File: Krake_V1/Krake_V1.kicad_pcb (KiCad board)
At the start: 4 copper layers, 107.5 x 102 mm, 60 parts, among them J1 Barrel_Jack_Switch_SMT, Q1 BSS138, U1 LM7805_TO220, U2 PCF8574AT_3_518, U3 LCD_20x4_Character-GPAD_SCH_L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

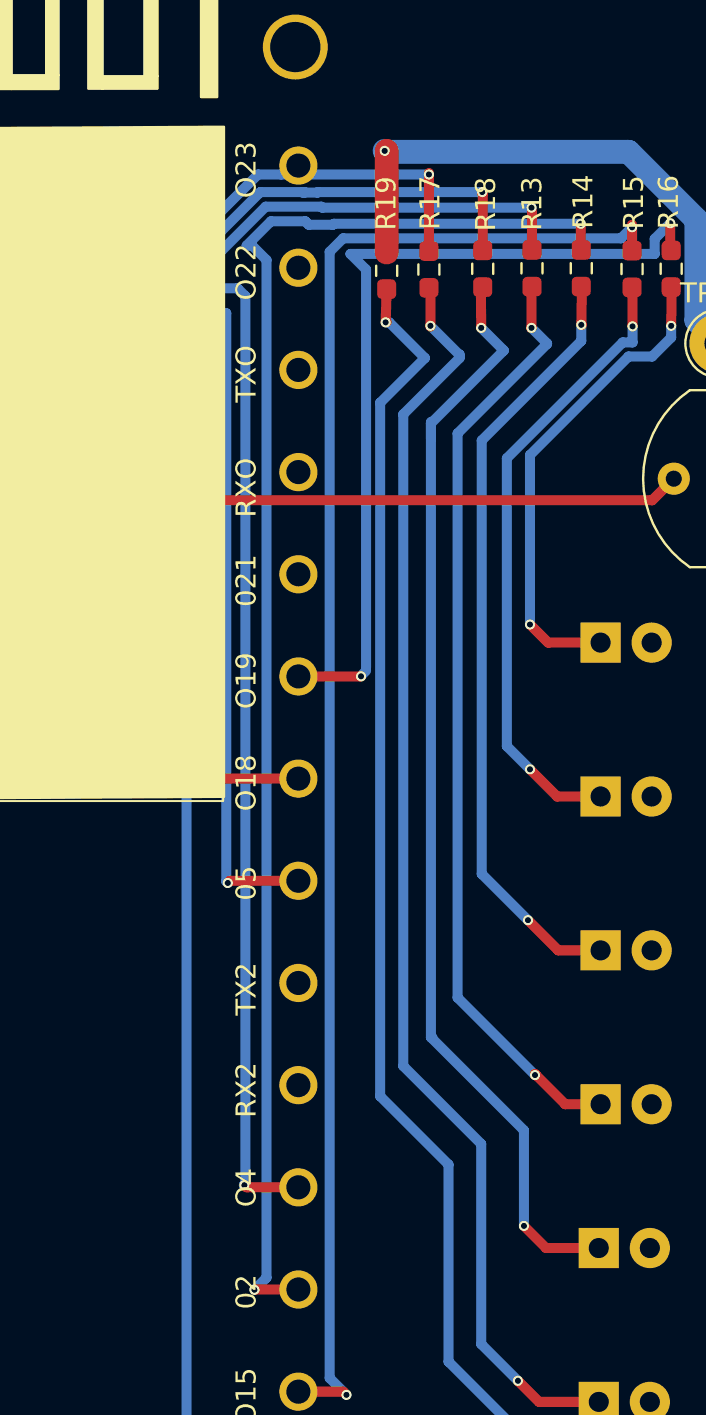
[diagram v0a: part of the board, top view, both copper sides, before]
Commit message: Placed the files for LCD debugging in a factory test file.
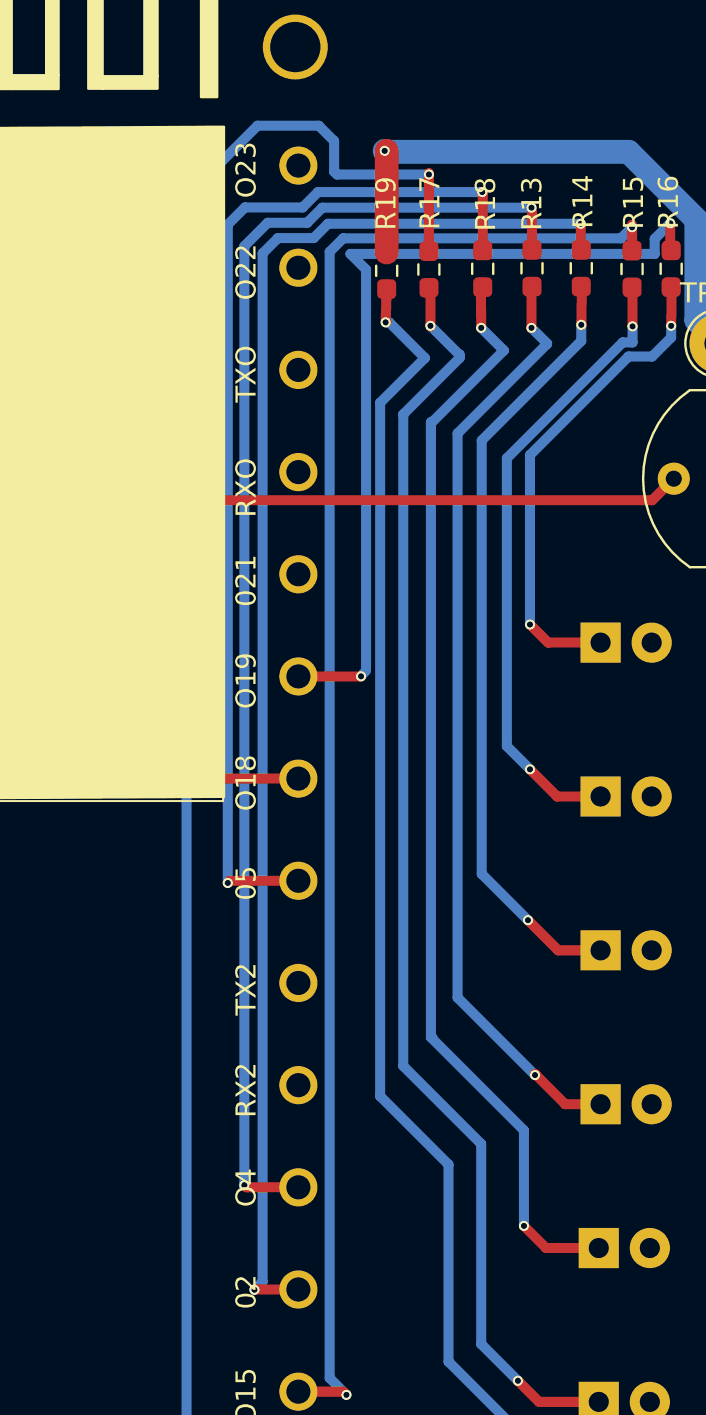
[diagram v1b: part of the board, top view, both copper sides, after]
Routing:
- net Net-(ESP1-O4): track 71.1 -> 66.5 mm
- net Net-(ESP1-O5): track 57.1 -> 52.5 mm
- net Net-(ESP1-O2): track 73.4 -> 71.6 mm
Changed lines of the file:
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@@
   (via (at 202.325 34.175) (size 0.5) (drill 0.3) (layers "F.Cu" "B.Cu") (net 31))
   (via (at 191 63.9) (size 0.5) (drill 0.3) (layers "F.Cu" "B.Cu") (net 31))
-  (segment (start 202.325 34.175) (end 194.975 34.175) (width 0.5) (layer "B.Cu") (net 31))
-  (segment (start 190.975 63.875) (end 191 63.9) (width 0.5) (layer "B.Cu") (net 31))
-  (segment (start 187.25 40.875) (end 188.55 42.175) (width 0.5) (layer "B.Cu") (net 31))
-  (segment (start 194.975 34.175) (end 193.828079 34.175) (width 0.5) (layer "B.Cu") (net 31))
-  (segment (start 190.975 42.5) (end 190.975 63.875) (width 0.5) (layer "B.Cu") (net 31))
-  (segment (start 188.875 42.5) (end 190.975 42.5) (width 0.5) (layer "B.Cu") (net 31))
-  (segment (start 188.55 42.175) (end 188.875 42.5) (width 0.5) (layer "B.Cu") (net 31))
-  (segment (start 193.828079 34.175) (end 187.25 40.753079) (width 0.5) (layer "B.Cu") (net 31))
-  (segment (start 187.25 40.753079) (end 187.25 40.875) (width 0.5) (layer "B.Cu") (net 31))
+  (segment (start 197.612 32.512) (end 196.85 31.75) (width 0.5) (layer "B.Cu") (net 31))
+  (segment (start 193.802 31.75) (end 191.625 33.927) (width 0.5) (layer "B.Cu") (net 31))
+  (segment (start 197.612 34.036) (end 197.612 32.512) (width 0.5) (layer "B.Cu") (net 31))
+  (segment (start 196.85 31.75) (end 193.802 31.75) (width 0.5) (layer "B.Cu") (net 31))
+  (segment (start 197.751 34.175) (end 197.612 34.036) (width 0.5) (layer "B.Cu") (net 31))
+  (segment (start 191.625 63.275) (end 191 63.9) (width 0.5) (layer "B.Cu") (net 31))
+  (segment (start 202.325 34.175) (end 197.751 34.175) (width 0.5) (layer "B.Cu") (net 31))
+  (segment (start 191.625 33.927) (end 191.625 63.275) (width 0.5) (layer "B.Cu") (net 31))
   (segment (start 195.835 69.2916) (end 192.4334 69.2916) (width 0.5) (layer "F.Cu") (net 32))
   (segment (start 192.4334 69.2916) (end 192.325 69.4) (width 0.5) (layer "F.Cu") (net 32))
@@
   (via (at 192.325 69.4) (size 0.5) (drill 0.3) (layers "F.Cu" "B.Cu") (net 32))
   (via (at 204.975 35.05) (size 0.5) (drill 0.3) (layers "F.Cu" "B.Cu") (net 32))
-  (segment (start 189.731971 41.075) (end 192.25 41.075) (width 0.5) (layer "B.Cu") (net 32))
-  (segment (start 192.25 69.325) (end 192.325 69.4) (width 0.5) (layer "B.Cu") (net 32))
-  (segment (start 196.125 35.075) (end 196.15 35.05) (width 0.5) (layer "B.Cu") (net 32))
-  (segment (start 196.810051 35.05) (end 196.785051 35.075) (width 0.5) (layer "B.Cu") (net 32))
-  (segment (start 193.943029 35.05) (end 188.825 40.168029) (width 0.5) (layer "B.Cu") (net 32))
-  (segment (start 196.785051 35.075) (end 196.05 35.075) (width 0.5) (layer "B.Cu") (net 32))
-  (segment (start 188.825 40.168029) (end 189.731971 41.075) (width 0.5) (layer "B.Cu") (net 32))
-  (segment (start 196.15 35.05) (end 193.943029 35.05) (width 0.5) (layer "B.Cu") (net 32))
+  (segment (start 196.810051 35.05) (end 196.046051 35.814) (width 0.5) (layer "B.Cu") (net 32))
+  (segment (start 196.046051 35.814) (end 193.179029 35.814) (width 0.5) (layer "B.Cu") (net 32))
+  (segment (start 192.325 36.668029) (end 192.325 69.4) (width 0.5) (layer "B.Cu") (net 32))
   (segment (start 204.975 35.05) (end 196.810051 35.05) (width 0.5) (layer "B.Cu") (net 32))
-  (segment (start 196.05 35.075) (end 196.125 35.075) (width 0.5) (layer "B.Cu") (net 32))
-  (segment (start 192.25 41.075) (end 192.25 69.325) (width 0.5) (layer "B.Cu") (net 32))
+  (segment (start 193.179029 35.814) (end 192.325 36.668029) (width 0.5) (layer "B.Cu") (net 32))
   (segment (start 150.8 62.225) (end 148.45 62.225) (width 0.5) (layer "F.Cu") (net 34))
   (via (at 148.45 62.225) (size 0.5) (drill 0.3) (layers "F.Cu" "B.Cu") (net 34))
@@
   (via (at 207.425 35.825) (size 0.5) (drill 0.3) (layers "F.Cu" "B.Cu") (net 35))
   (via (at 193.15 84.425) (size 0.5) (drill 0.3) (layers "F.Cu" "B.Cu") (net 35))
-  (segment (start 190.15 39.832979) (end 192.807979 39.832979) (width 0.5) (layer "B.Cu") (net 35))
-  (segment (start 194.207979 35.775) (end 190.15 39.832979) (width 0.5) (layer "B.Cu") (net 35))
-  (segment (start 196.975 35.775) (end 194.207979 35.775) (width 0.5) (layer "B.Cu") (net 35))
+  (segment (start 193.15 37.736) (end 193.15 84.4) (width 0.5) (layer "B.Cu") (net 35))
+  (segment (start 194.31 36.576) (end 193.15 37.736) (width 0.5) (layer "B.Cu") (net 35))
+  (segment (start 207.425 35.825) (end 197.025 35.825) (width 0.5) (layer "B.Cu") (net 35))
   (segment (start 193.15 84.4) (end 193.15 84.425) (width 0.5) (layer "B.Cu") (net 35))
+  (segment (start 196.274 36.576) (end 194.31 36.576) (width 0.5) (layer "B.Cu") (net 35))
   (segment (start 193.15 84.425) (end 193.125 84.425) (width 0.5) (layer "B.Cu") (net 35))
-  (segment (start 193.2 40.225) (end 193.2 84.35) (width 0.5) (layer "B.Cu") (net 35))
-  (segment (start 193.2 84.35) (end 193.15 84.4) (width 0.5) (layer "B.Cu") (net 35))
-  (segment (start 207.425 35.825) (end 197.025 35.825) (width 0.5) (layer "B.Cu") (net 35))
-  (segment (start 192.807979 39.832979) (end 193.2 40.225) (width 0.5) (layer "B.Cu") (net 35))
+  (segment (start 197.025 35.825) (end 196.274 36.576) (width 0.5) (layer "B.Cu") (net 35))
   (segment (start 193.125 84.425) (end 193.15 84.4) (width 0.5) (layer "B.Cu") (net 35))
-  (segment (start 197.025 35.825) (end 196.975 35.775) (width 0.5) (layer "B.Cu") (net 35))
   (segment (start 209.9 37.925) (end 209.875 37.9) (width 0.5) (layer "F.Cu") (net 36))
   (segment (start 193.6634 89.6116) (end 193.65 89.625) (width 0.5) (layer "F.Cu") (net 36))
@@
   (via (at 209.875 36.625) (size 0.5) (drill 0.3) (layers "F.Cu" "B.Cu") (net 36))
   (via (at 193.65 89.625) (size 0.5) (drill 0.3) (layers "F.Cu" "B.Cu") (net 36))
-  (segment (start 193.536777 37.711777) (end 194.25 38.425) (width 0.5) (layer "B.Cu") (net 36))
-  (segment (start 209.875 36.625) (end 197.6 36.625) (width 0.5) (layer "B.Cu") (net 36))
-  (segment (start 194.470477 36.502451) (end 193.261151 37.711777) (width 0.5) (layer "B.Cu") (net 36))
-  (segment (start 193.261151 37.711777) (end 193.536777 37.711777) (width 0.5) (layer "B.Cu") (net 36))
-  (segment (start 196.353272 36.675) (end 196.180723 36.502451) (width 0.5) (layer "B.Cu") (net 36))
-  (segment (start 197.55 36.675) (end 196.353272 36.675) (width 0.5) (layer "B.Cu") (net 36))
-  (segment (start 196.180723 36.502451) (end 194.470477 36.502451) (width 0.5) (layer "B.Cu") (net 36))
-  (segment (start 194.25 38.425) (end 194.25 89.025) (width 0.5) (layer "B.Cu") (net 36))
-  (segment (start 194.25 89.025) (end 193.65 89.625) (width 0.5) (layer "B.Cu") (net 36))
-  (segment (start 197.6 36.625) (end 197.55 36.675) (width 0.5) (layer "B.Cu") (net 36))
+  (segment (start 194.056 89.219) (end 193.65 89.625) (width 0.5) (layer "B.Cu") (net 36))
+  (segment (start 194.056 38.1) (end 194.056 89.219) (width 0.5) (layer "B.Cu") (net 36))
+  (segment (start 196.596 37.338) (end 194.818 37.338) (width 0.5) (layer "B.Cu") (net 36))
+  (segment (start 197.309 36.625) (end 196.596 37.338) (width 0.5) (layer "B.Cu") (net 36))
+  (segment (start 194.818 37.338) (end 194.056 38.1) (width 0.5) (layer "B.Cu") (net 36))
+  (segment (start 209.875 36.625) (end 197.309 36.625) (width 0.5) (layer "B.Cu") (net 36))
   (segment (start 212.425 37.9625) (end 212.425 36.675) (width 0.5) (layer "F.Cu") (net 37))
   (segment (start 195.835 94.6916) (end 198.0666 94.6916) (width 0.5) (layer "F.Cu") (net 37))
